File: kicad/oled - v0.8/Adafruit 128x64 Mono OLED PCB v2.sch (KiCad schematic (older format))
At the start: 59 parts, among them SW1 SW_Reed, SW2 SW_Reed, SW3 SW_Push, SW4 SW_Push, SW5 SW_Push, SW6 SW_Reed, U1 UG-2864HSWEG01, U3 NRF52832-QFAA-R, Y1 32MHz

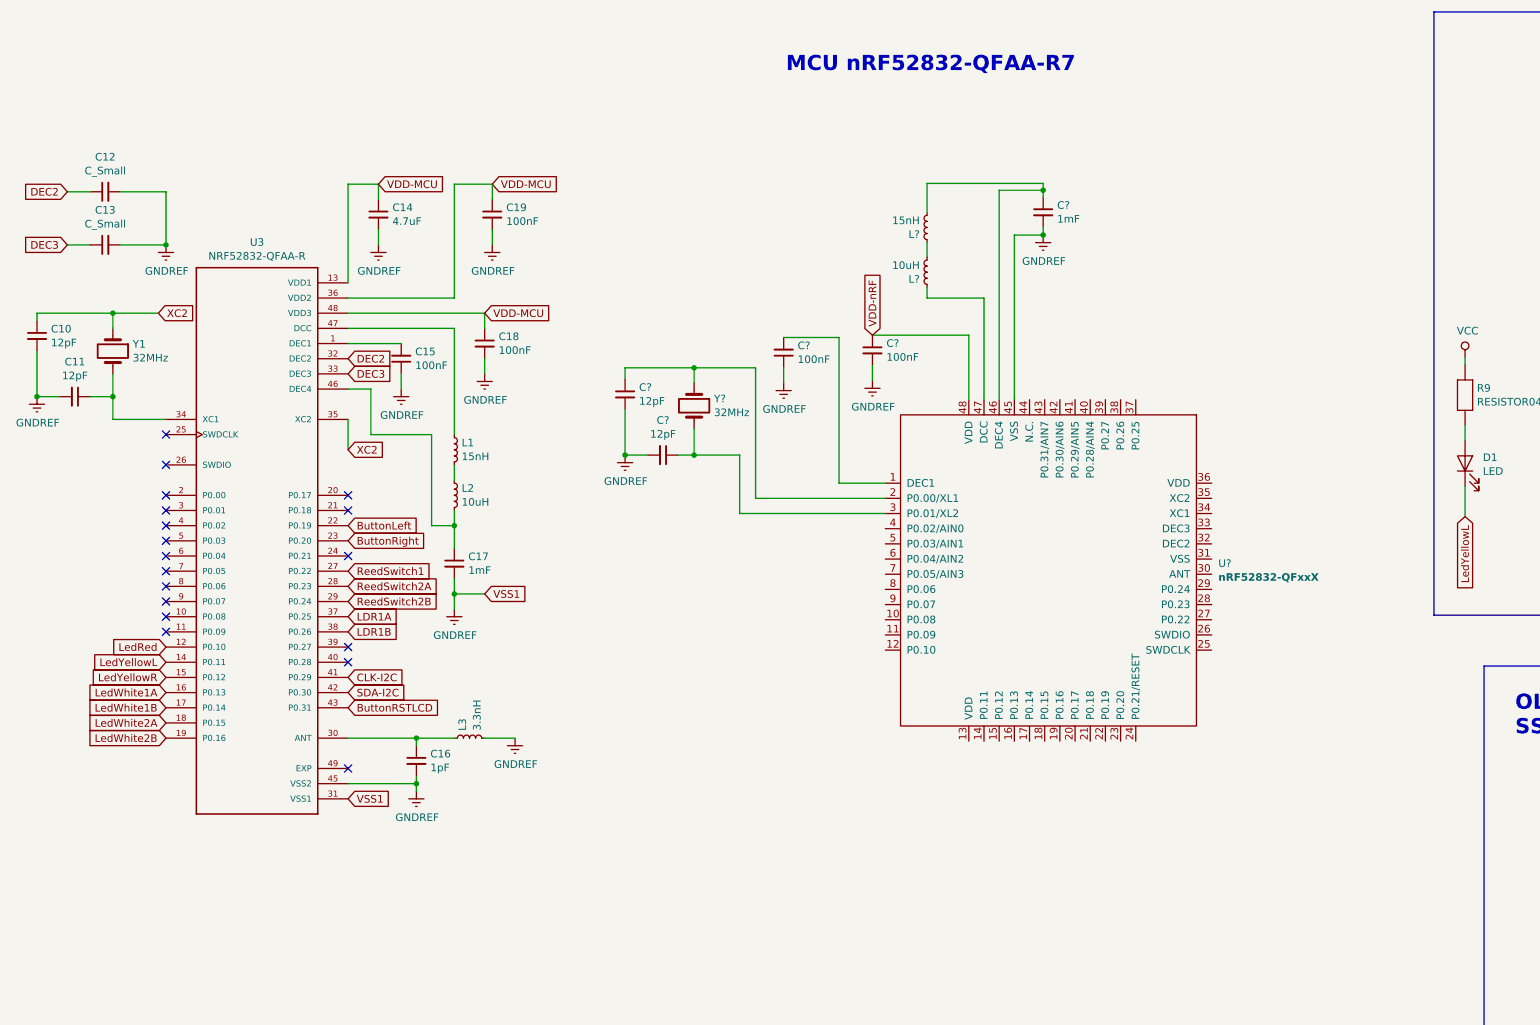
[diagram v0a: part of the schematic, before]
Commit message: Versão 8 do projeto. nRF finalizada. Verificar o LCD.
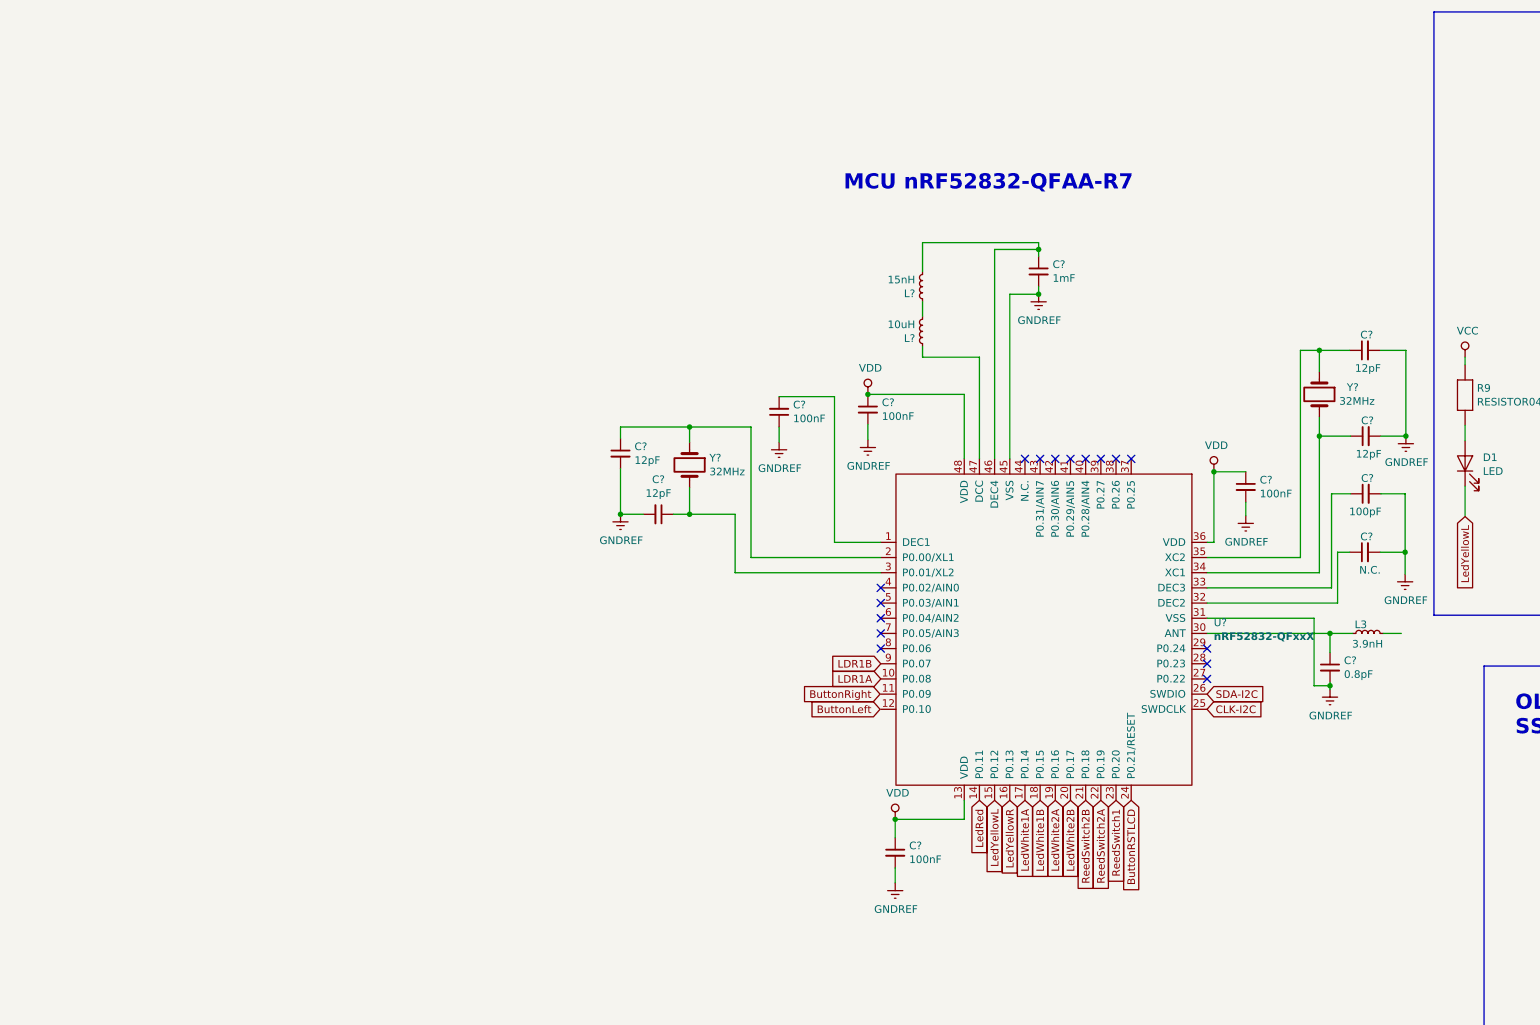
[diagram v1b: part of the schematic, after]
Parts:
- removed C10, C11: 12pF, symbol Device:C_Small
- removed C12, C13: C_Small, symbol Device:C_Small
- removed C14: 4.7uF, symbol Device:C_Small
- removed C15, C18, C19: 100nF, symbol Device:C_Small
- removed C16: 1pF, symbol Device:C_Small
- removed C17: 1mF, symbol Device:C_Small
- removed L1: 15nH, symbol Device:L_Small
- removed L2: 10uH, symbol Device:L_Small
- removed U3: NRF52832-QFAA-R, QFN40P600X600X90-49N, symbol Adafruit-128x64-Mono-OLED-PCB-v2-rescue:NRF52832-QFAA-R-MCU_Nordic
- removed Y1: 32MHz, symbol Device:Crystal
- added C? (x2): 100nF, symbol Device:C_Small
- added C? (x2): 12pF, symbol Device:C_Small
- added C?: 100pF, symbol Device:C_Small
- added C?: N.C., symbol Device:C_Small
- added C?: 0.8pF, symbol Device:C_Small
- added Y?: 32MHz, symbol Device:Crystal
- L3: value 3.3nH -> 3.9nH
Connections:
- net VDD-nRF is gone; now on net VDD: C?.1, U?.48 (VDD)
- net ButtonRSTLCD: now also U?.24 (P0.21/RESET)
- net CLK-I2C: now also U?.25 (SWDCLK)
- net GNDREF: now also U?.31 (VSS), C?.2, C?.2, C?.2, C?.2, C?.2, C?.2, C?.2; no longer L3.2
- net LDR1A: now also U?.10 (P0.08)
- net LDR1B: now also U?.9 (P0.07)
- net LedRed: now also U?.14 (P0.11)
- net LedWhite1A: now also U?.17 (P0.14)
- net LedWhite1B: now also U?.18 (P0.15)
- net LedWhite2A: now also U?.19 (P0.16)
- net LedWhite2B: now also U?.20 (P0.17)
- net LedYellowL: now also U?.15 (P0.12)
- net LedYellowR: now also U?.16 (P0.13)
- net ReedSwitch1: now also U?.23 (P0.20)
- net ReedSwitch2A: now also U?.22 (P0.19)
- net ReedSwitch2B: now also U?.21 (P0.18)
- net SDA-I2C: now also U?.26 (SWDIO)
- net at L3.1: now also U?.30 (ANT), C?.1
- net VDD: now reaches U?.13 (VDD)
- net VDD: now also U?.36 (VDD), C?.1, C?.1
- net at U?.32 (DEC2): now also C?.1
- net at U?.33 (DEC3): now also C?.1
- net at U?.34 (XC1): now also C?.1, Y?.2
- net at U?.35 (XC2): now also C?.1, Y?.1
- no-connect marks 41 -> 39
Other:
- moved on the sheet: C?, L3, L?, U?, Y?

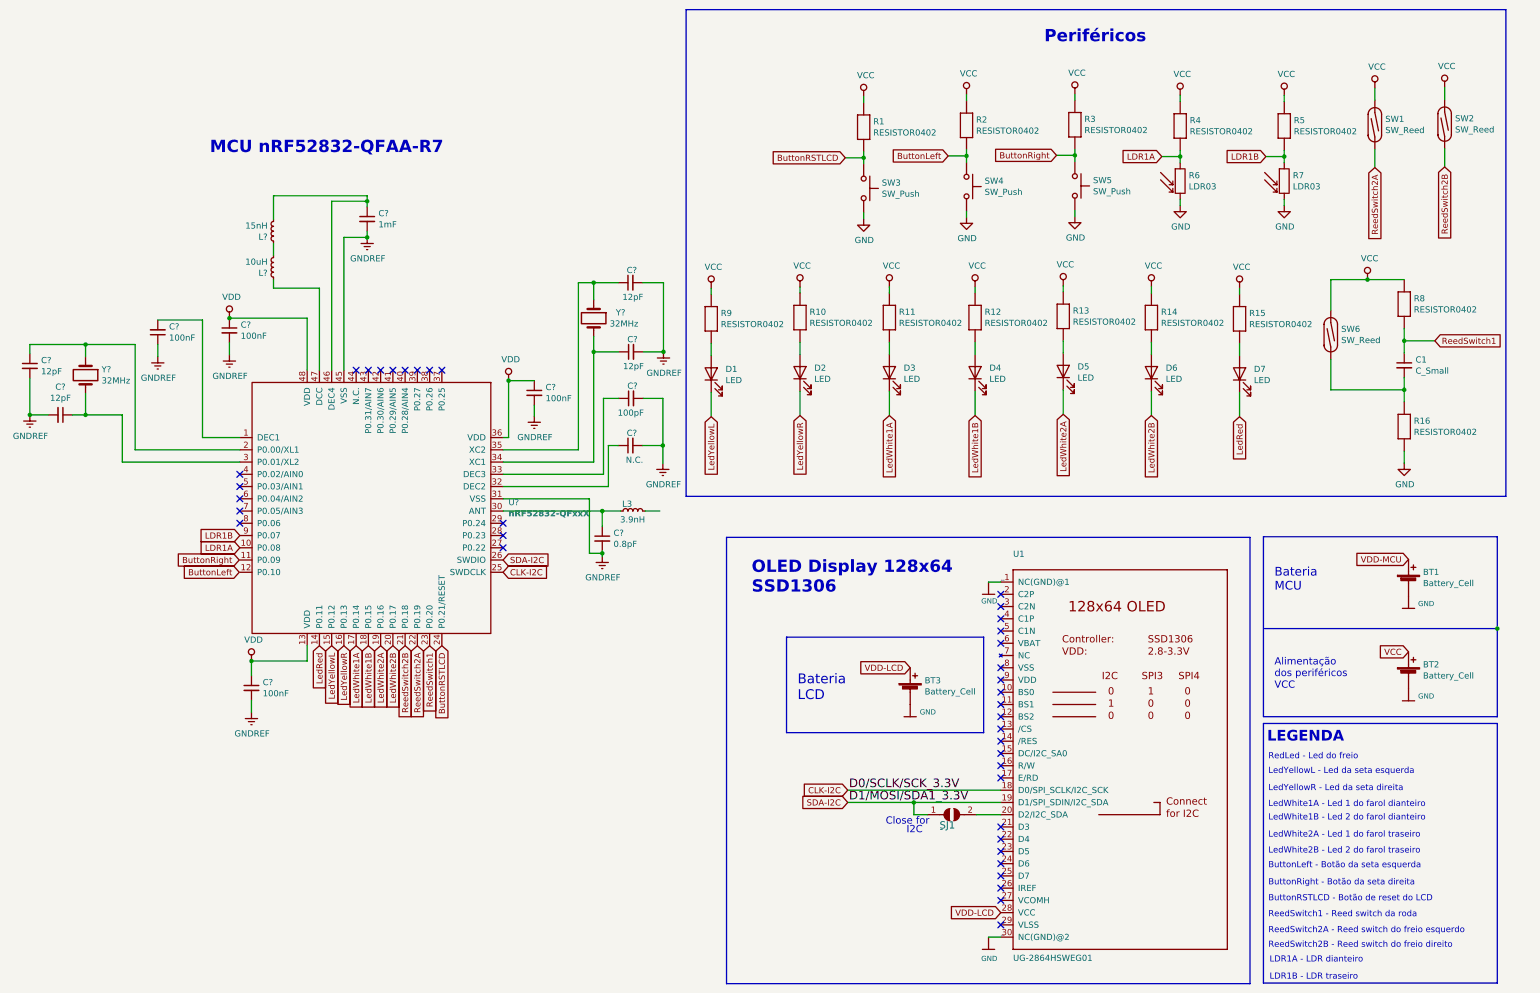
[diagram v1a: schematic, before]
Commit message: Atualizando v0.8
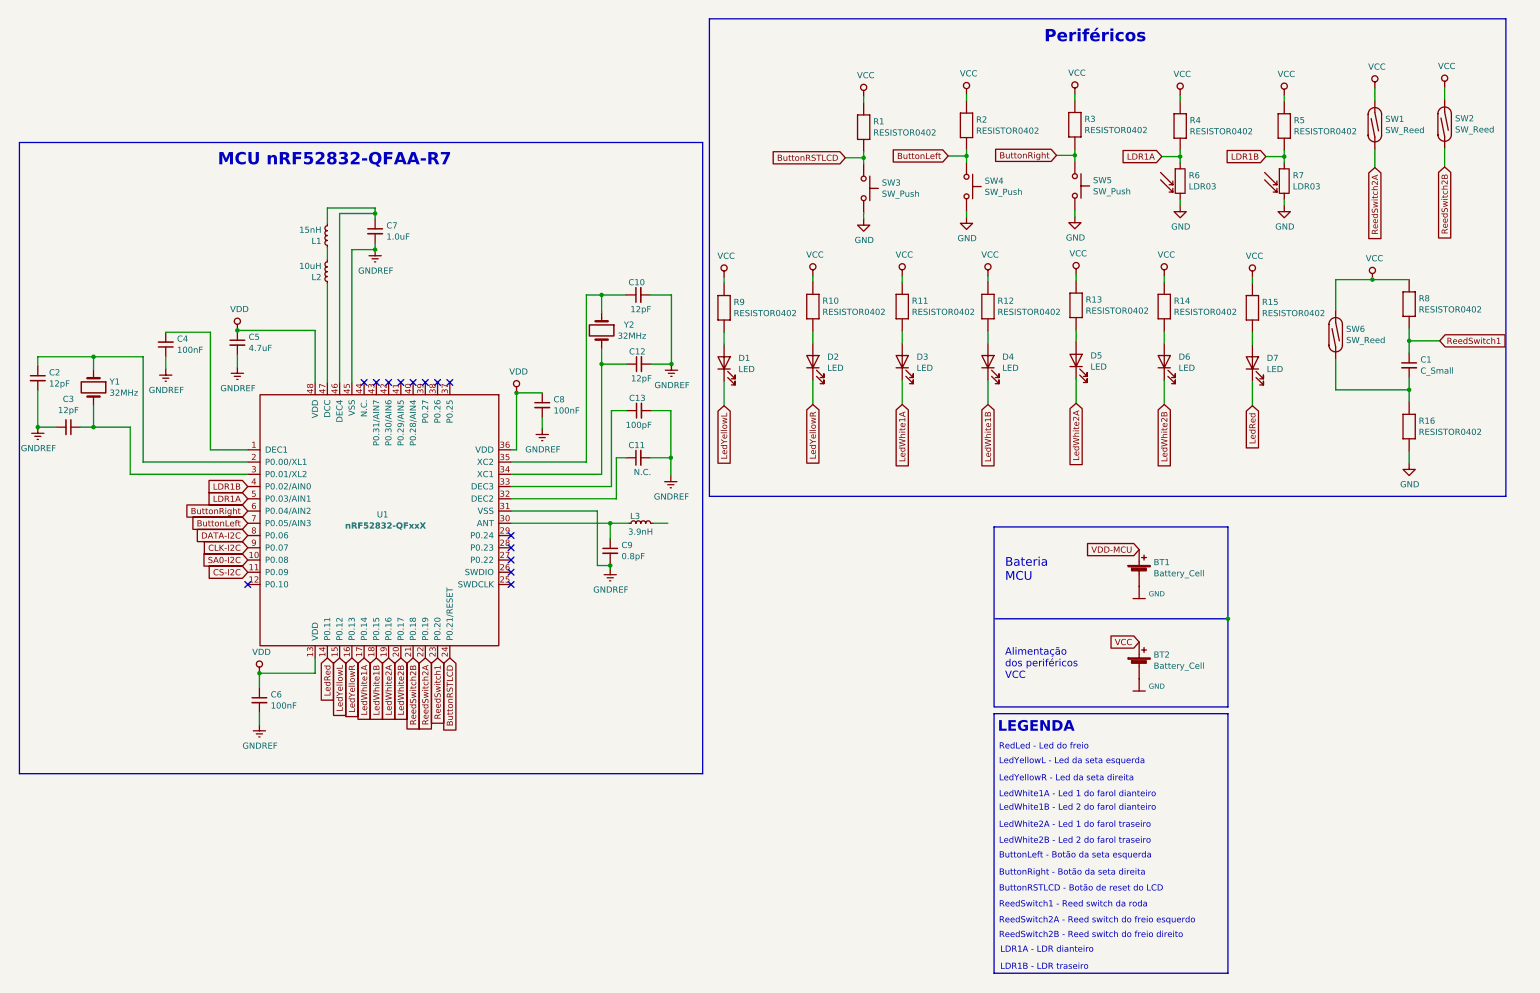
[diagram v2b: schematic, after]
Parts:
- removed BT3: Battery_Cell, symbol Device:Battery_Cell
- removed SJ1: -, Adafruit 128x64 Mono OLED PCB v2:SOLDERJUMPER_REFLOW_NOPASTE, symbol Adafruit_128x64_Mono_OLED_PCB_v2-eagle-import:SOLDERJUMPERREFLOW_NOPASTE
- removed U1: UG-2864HSWEG01, Adafruit 128x64 Mono OLED PCB v2:UG-2864HSWEG01_0.96IN_WRAPAROUND, symbol Adafruit_128x64_Mono_OLED_PCB_v2-eagle-import:DISP_OLED_UG-2864HSWEG010.96"
- BT1, BT2: footprint (none) -> Battery:Battery_Panasonic_CR2032-VS1N_Vertical_CircularHoles
- C10, C11, C12, C13, C2, C3, C4, C6, C8, C9: renamed from C?; footprint (none) -> Capacitor_SMD:C_0402_1005Metric
- C5: renamed from C?; value 100nF -> 4.7uF; footprint (none) -> Capacitor_SMD:C_0402_1005Metric
- C7: renamed from C?; value 1mF -> 1.0uF; footprint (none) -> Capacitor_SMD:C_0402_1005Metric
- L1, L2: renamed from L?; footprint (none) -> Inductor_SMD:L_0402_1005Metric
- L3: footprint (none) -> Inductor_SMD:L_0402_1005Metric
- R1, R10, R11, R12, R13, R14, R15, R16, R2, R3, R4, R5, R8, R9: footprint (none) -> Resistor_SMD:R_0402_1005Metric
- gave numbers to parts that had none: 3
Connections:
- net ButtonLeft: now also U1.7 (P0.05/AIN3)
- net ButtonRight: now also U1.6 (P0.04/AIN2)
- net CLK-I2C: now also U1.9 (P0.07); no longer U1.25 (SWDCLK)
- net LDR1A: now also U1.5 (P0.03/AIN1); no longer U1.10 (P0.08)
- net LDR1B: now also U1.4 (P0.02/AIN0); no longer U1.9 (P0.07)
- net CS-I2C: now reaches U1.11 (P0.09)
- net DATA-I2C: now reaches U1.8 (P0.06)
- net SDA-I2C: no longer names the net of U1.26 (SWDIO)
- new net SA0-I2C: U1.10 (P0.08)
- no-connect marks 39 -> 14
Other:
- note removed: "Bateria\nLCD"
- note removed: "Close for"
- note removed: "I2C"
- note removed: "OLED Display 128x64\nSSD1306"
- moved on the sheet: BT1, BT2, C1, C10, C11, C12, C13, C2, C3, C4, C5, C6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
